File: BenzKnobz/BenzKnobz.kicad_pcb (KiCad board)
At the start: 2 copper layers, 1.3 x 11.1 mm, 115 parts, among them J1 Barrel_Jack, J10 I2C_STANDARDJS-1MM, J2 MIDI OUT, J3 MIDI IN, J4 MJ-3502, J5 MJ-3502, J6 MJ-3502, J7 MJ-3502, J8 MJ-3502, J9 MJ-3502, SW1 SW_MEC_5E, SW2 SW_MEC_5E, SW3 SW_MEC_5E, SW4 SW_MEC_5E, SW5 SW_MEC_5E, SW6 SW_MEC_5E, U1 teensy 4.0, U10 6N138, U2 TXB0108DQSR, U3 74HC4051, U4 74HC4051, U5 74HC4051, U6 74HC4051, U7 74HC4051, U8 74HC4051, U9 74HC4051

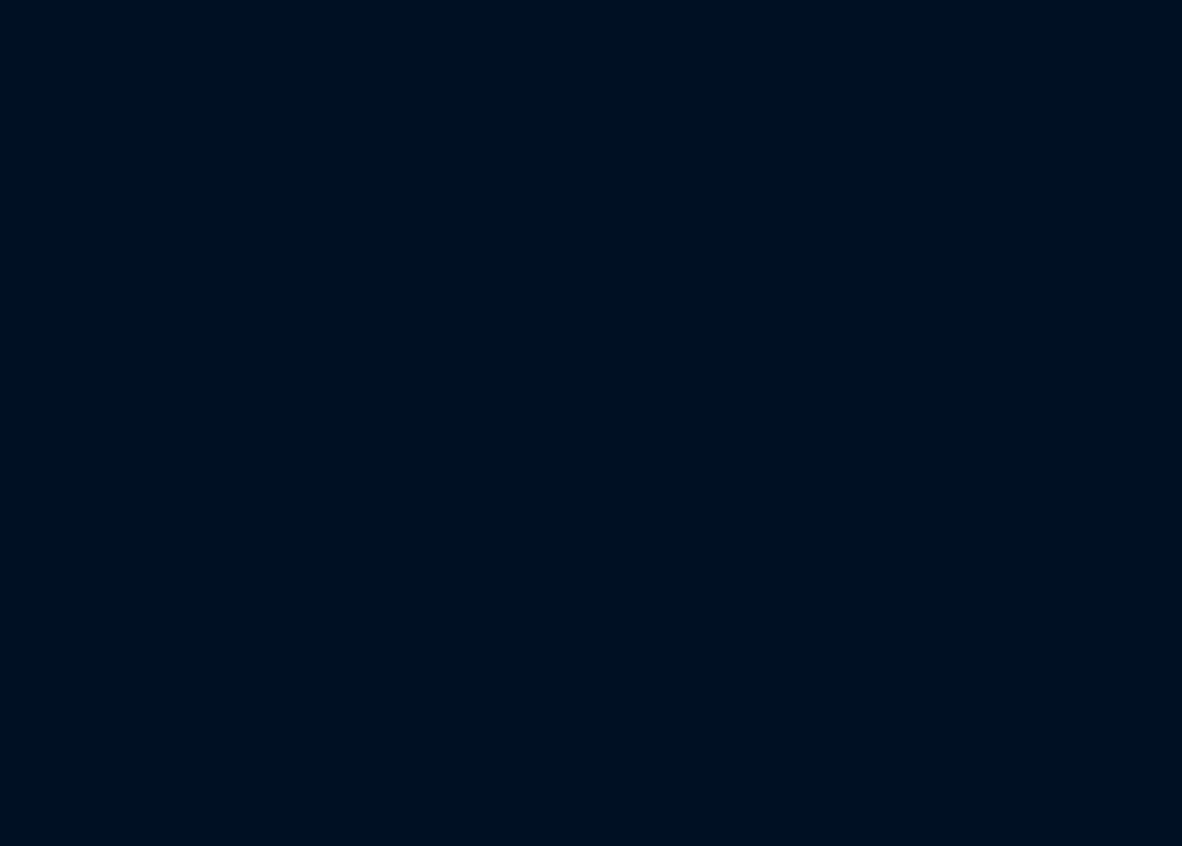
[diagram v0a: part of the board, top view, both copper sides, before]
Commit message: circuit/board
finalizing power regulation
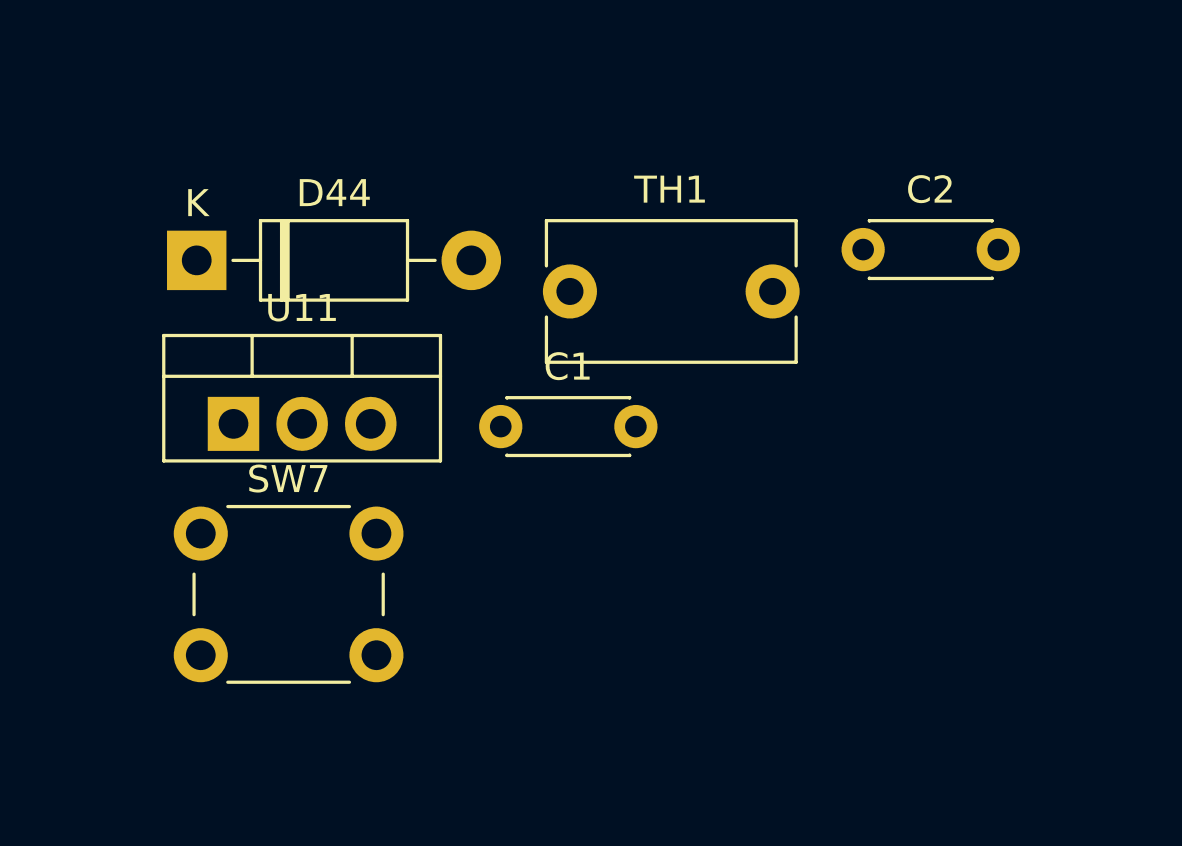
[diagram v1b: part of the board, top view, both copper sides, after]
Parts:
- added C1: CAP_CERAMIC0402, Capacitor_THT:C_Disc_D4.3mm_W1.9mm_P5.00mm, F.Cu at (215.9, 111.8)
- added C2: CAP_CERAMIC0402, Capacitor_THT:C_Disc_D4.3mm_W1.9mm_P5.00mm, F.Cu at (229.3, 105.2)
- added D44: 1N4007, Diode_THT:D_DO-41_SOD81_P10.16mm_Horizontal, F.Cu at (204.7, 105.6)
- added SW7: SW_Push_SPDT, Button_Switch_THT:SW_PUSH_6mm, F.Cu at (204.8, 115.7)
- added TH1: Thermistor, Capacitor_THT:C_Disc_D9.0mm_W5.0mm_P7.50mm, F.Cu at (218.5, 106.8)
- added U11: LM317_TO-220, Package_TO_SOT_THT:TO-220-3_Vertical, F.Cu at (206.0, 111.7)
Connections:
- J1 pad 1: 5VDC -> +5V
- U1 pad VIN: 5VDC -> Net-(U1-PadVIN)
- U2 pad 16: 5VDC -> Net-(U1-PadVIN)
